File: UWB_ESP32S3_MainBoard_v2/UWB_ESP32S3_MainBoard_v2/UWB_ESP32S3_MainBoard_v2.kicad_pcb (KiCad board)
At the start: 2 copper layers, 90 x 90 mm, 42 parts, among them J1 ESP32_S3_2, J10 MP1584EN_IN, J11 MP1584EN_OUT, J12 MINI360_IN, J13 MINI360_OUT, J14 VBAT, J15 MOTOR_L, J16 MOTOR_R, J2 ESP32_S3_1, J3 BNO085, J4 DRV8833_L_OUT, J5 DRV8833_L_IN, J6 DRV8833_R_OUT, J7 DRV8833_R_IN, J8 TAU_1201, J9 ESP32_UWBAOA_UART

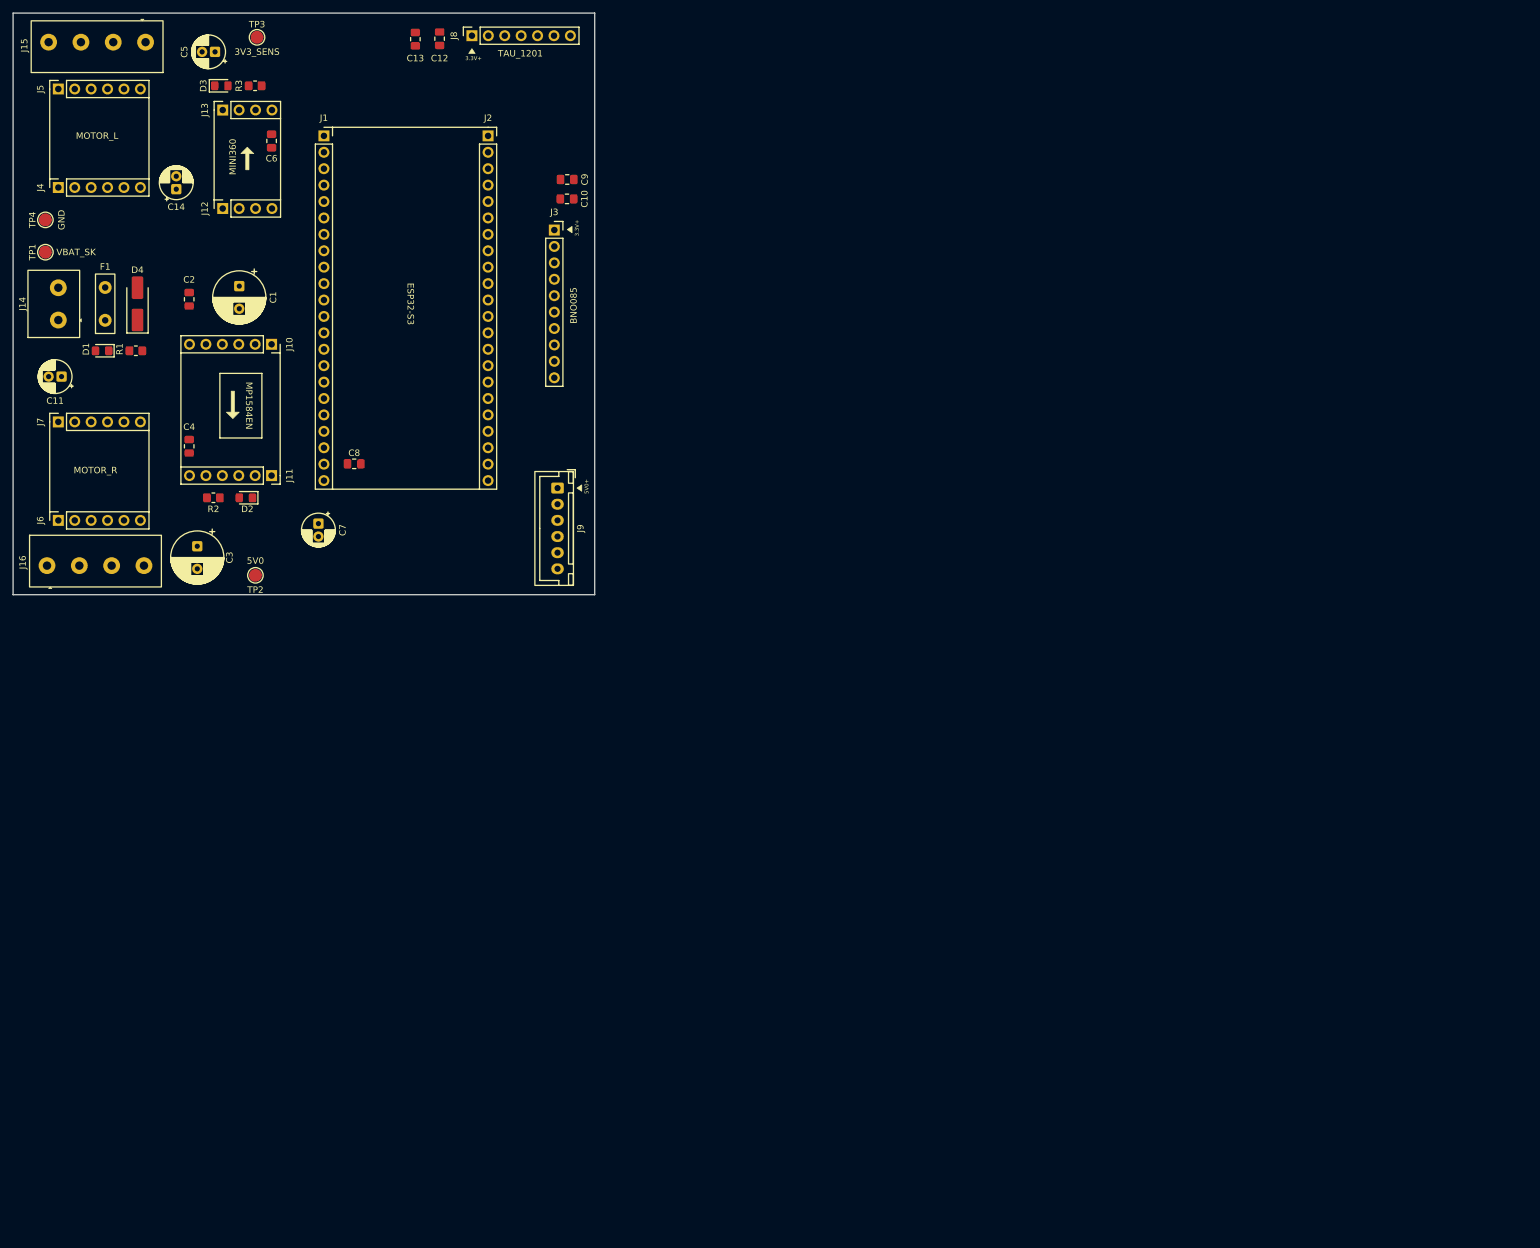
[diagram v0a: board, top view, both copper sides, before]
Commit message: 테스트
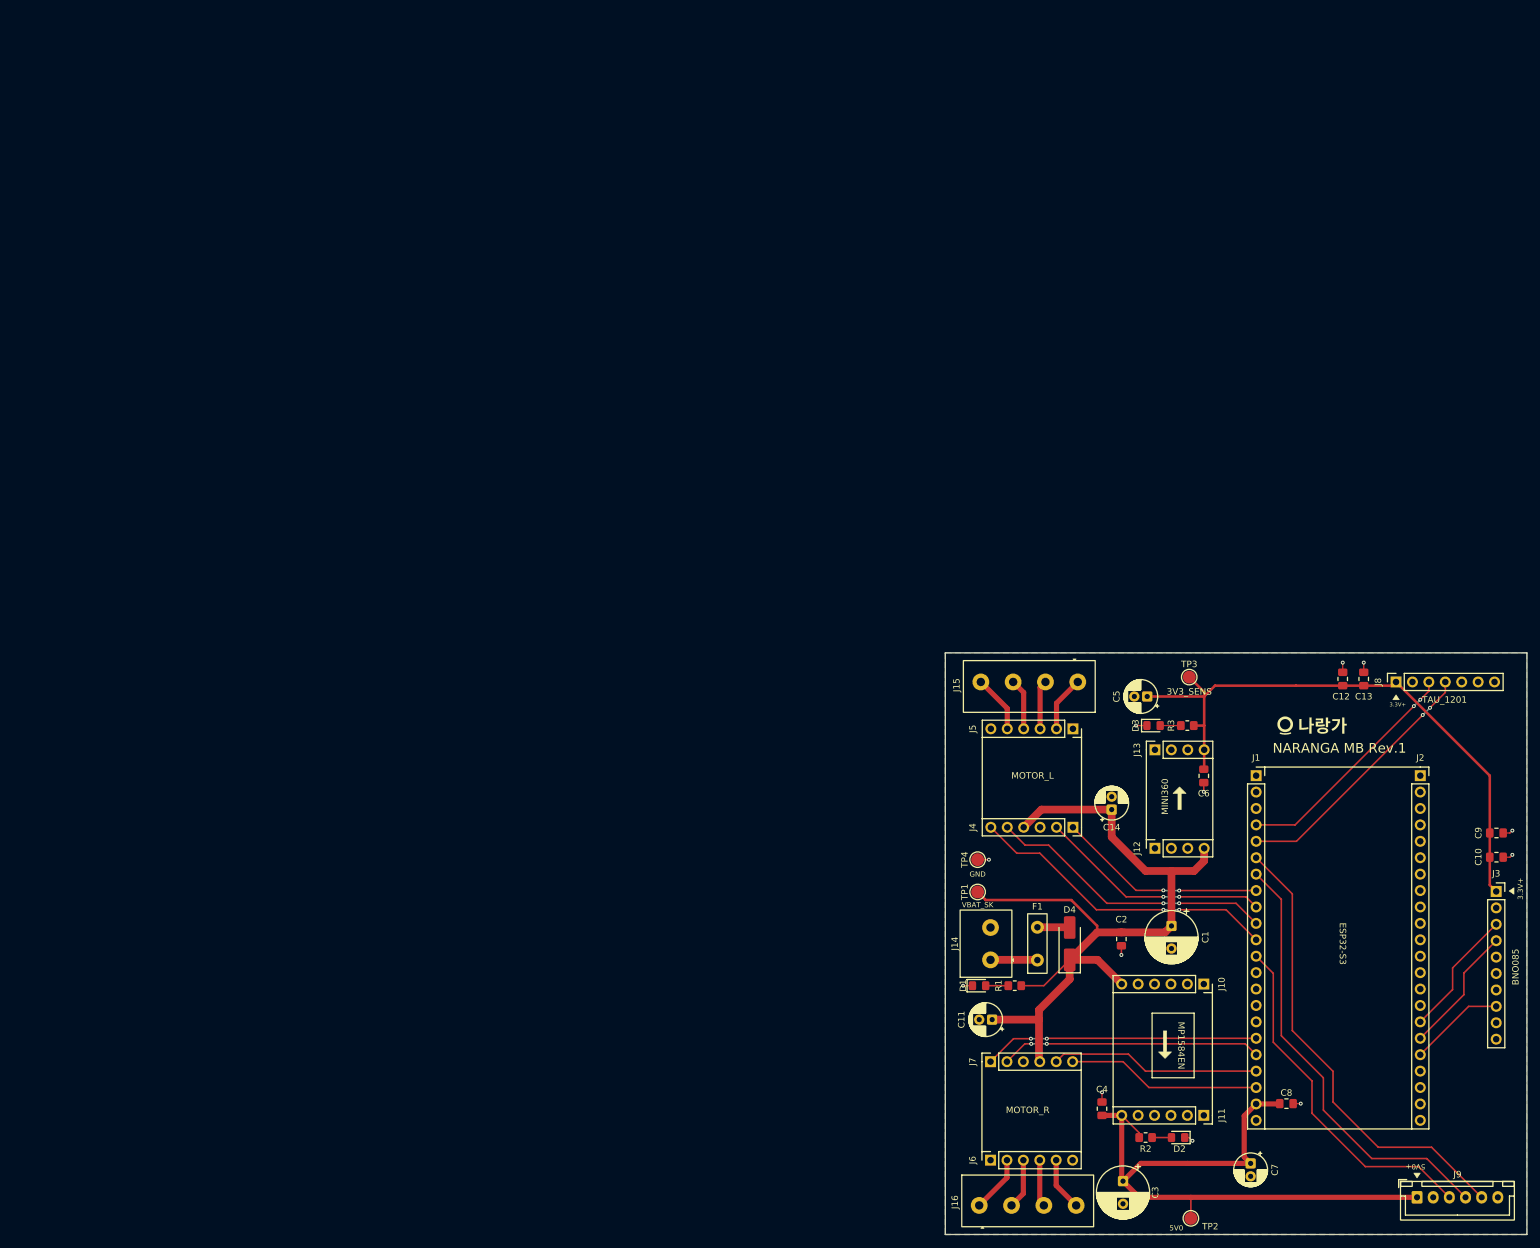
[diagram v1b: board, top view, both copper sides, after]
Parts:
- added G***: LOGO, 10000_custom_Library:NARANGA_logo, F.Cu at (156.0, 65.2)
- moved J4 185.6 mm to (119.0, 81.0), turned to -90 degrees
- moved J5 185.6 mm to (119.0, 65.8), turned to -90 degrees
- moved J3 178.1 mm to (184.5, 90.9)
- moved C13 177.0 mm to (164.0, 58.0)
- moved C10 176.2 mm to (184.5, 85.6)
- moved C9 175.8 mm to (184.5, 81.9)
- moved TP2 175.6 mm to (137.2, 141.5)
- moved C5 175.4 mm to (130.5, 60.8)
- moved C11 175.0 mm to (106.5, 110.8)
- moved C1 175.0 mm to (134.2, 96.2)
- moved C2 175.0 mm to (126.5, 98.3)
- moved C7 175.0 mm to (146.5, 133.0)
- moved C8 175.0 mm to (152.0, 123.8)
- moved D2 175.0 mm to (135.3, 129.0)
- moved D3 175.0 mm to (131.5, 65.2)
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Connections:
- net GND renamed /GND
- J15 pad 1: /LR_B -> /LF_A
- J15 pad 2: /LR_A -> /LF_B
- J15 pad 3: /LF_B -> /LR_A
- J15 pad 4: /LF_A -> /LR_B
- J3 pad 3: /IO47 -> /IO48
- J3 pad 4: /IO48 -> /IO47
- J5 pad 1: /EEP -> unconnected-(J5-Pin_1-Pad1)
- J5 pad 6: /ULT -> unconnected-(J5-Pin_6-Pad6)
- J8 pad 3: /IO5 -> /IO4
- J8 pad 4: /IO4 -> /IO5
- J9 pad 3: /IO6 -> /IO8
- J9 pad 5: /IO8 -> /IO6
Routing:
- net /VBAT_SK: track 0.00 -> 130.0 mm
- net /5V0: track 0.00 -> 102.6 mm
- net /3V3_SENS: track 0.00 -> 95.1 mm
- net /IO6: track 0.00 -> 71.8 mm
- net /IO7: track 0.00 -> 68.4 mm
- net /IO8: track 0.00 -> 54.5 mm
- net /IO18: track 0.00 -> 48.3 mm, vias 0 -> 2
- net /IO17: track 0.00 -> 44.7 mm, vias 0 -> 2
- net /IO11: track 0.00 -> 42.6 mm, vias 0 -> 2
- net /IO5: track 0.00 -> 40.4 mm, vias 0 -> 2
- net /IO12: track 0.00 -> 40.4 mm, vias 0 -> 2
- net /IO4: track 0.00 -> 36.7 mm, vias 0 -> 2
- net /IO16: track 0.00 -> 36.0 mm, vias 0 -> 2
- net /IO13: track 0.00 -> 32.5 mm
- net /IO15: track 0.00 -> 32.4 mm, vias 0 -> 2
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- added copper zone on B.Cu, net /GND
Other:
- board text added: "NARANGA MB Rev.1"
